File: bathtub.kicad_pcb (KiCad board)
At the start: 2 copper layers, 91.4 x 71.1 mm, 29 parts, among them J1 Screw_Terminal_01x03 - Hot wa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, J2 Screw_Terminal_01x03 - Cold w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, J3 Screw_Terminal_01x02, J4 Screw_Terminal_01x03 - Inputs, J5 Barrel_Jack, Q1 2N2219, Q2 2N2219, SW1 SW_Push, SW2 SW_Push

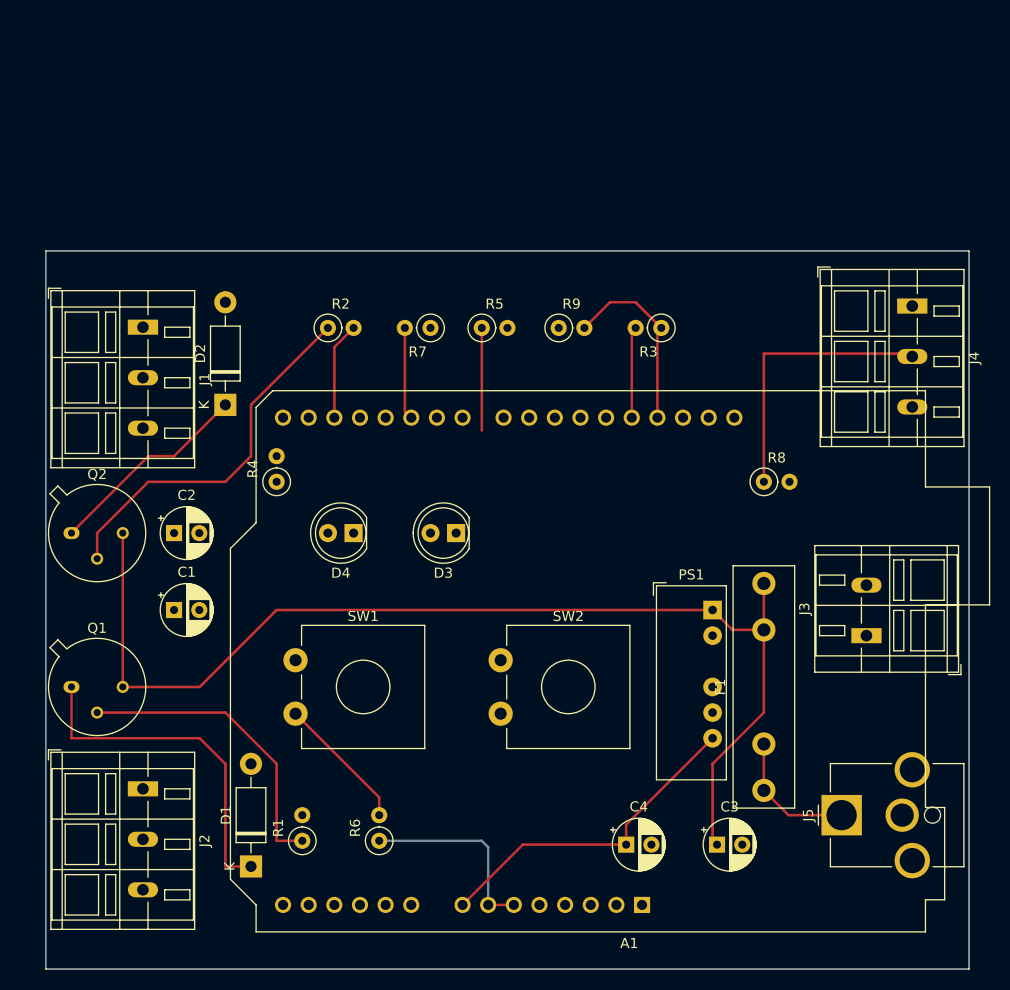
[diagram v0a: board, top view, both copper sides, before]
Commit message: feat: version 1.  Sent out for review
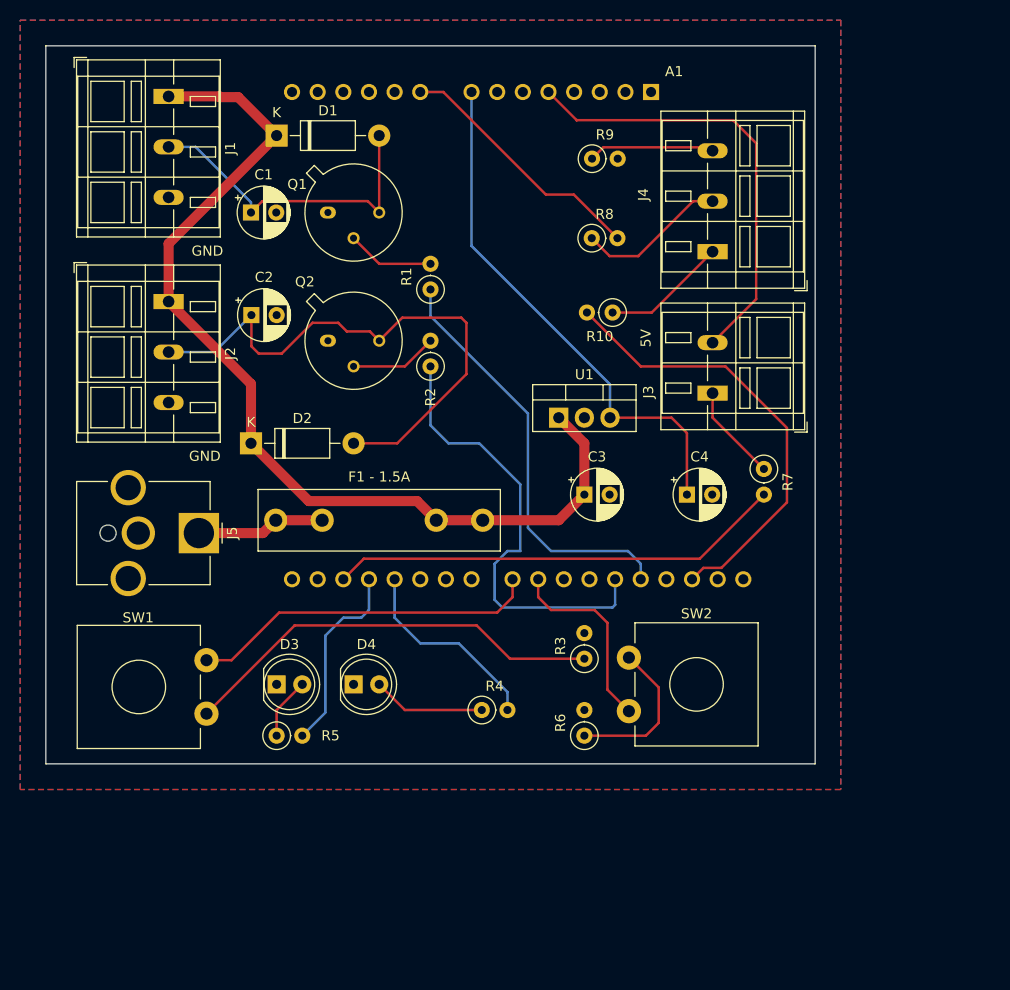
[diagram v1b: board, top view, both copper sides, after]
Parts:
- removed F1: Slow Blow Fuse - 1.5A, Fuse:Fuseholder_Littelfuse_100_series_5x20mm
- removed PS1: IH2405S, Converter_DCDC:Converter_DCDC_XP_POWER-IHxxxxS_THT
- added F1 - 1.5A: Slow Blow Fuse - 1.5A, Fuse:Fuseholder_Littelfuse_100_series_5x20mm, F.Cu at (119.3, 95.2)
- added R10: .01, Resistor_THT:R_Axial_DIN0207_L6.3mm_D2.5mm_P2.54mm_Vertical, F.Cu at (152.7, 74.7)
- added U1: L7805CV, Package_TO_SOT_THT:TO-220-3_Vertical, F.Cu at (147.3, 85.1)
- A1: moved to B.Cu
- C1, C2: value 0.1uF -> 0.01uF
- J1: value Screw_Terminal_01x03 - Hot water -> Screw_Terminal_01x03
- J2: value Screw_Terminal_01x03 - Cold water -> Screw_Terminal_01x03
- J3: value Screw_Terminal_01x02 -> Terminal_01x02
- J4: value Screw_Terminal_01x03 - Inputs -> Terminal 01x03 - Inputs
- R1, R2: value 250 ohms -> 250
- R3, R6: value 200ohm -> 200
- R4, R5: value 100ohm -> 220
- moved A1 80.5 mm to (156.5, 52.8)
- moved D1 72.4 mm to (119.4, 57.1), turned to 0 degrees
- moved J5 69.5 mm to (111.7, 96.5), turned to -90 degrees
- moved R1 56.1 mm to (134.6, 72.4)
- moved Q1 53.4 mm to (124.5, 64.8)
- moved J2 48.3 mm to (108.7, 73.6)
- moved R5 45.2 mm to (119.4, 116.6)
- moved C1 40.1 mm to (116.8, 64.8)
- moved C3 37.1 mm to (149.9, 92.7)
- moved R7 35.9 mm to (167.6, 90.2), turned to -90 degrees
- moved C4 35.2 mm to (160.0, 92.7)
- moved R3 33.6 mm to (149.9, 109.0), turned to 90 degrees
- moved Q2 31.7 mm to (124.5, 77.5)
- moved R4 30.4 mm to (139.7, 114.0), turned to 0 degrees
- moved R8 29.5 mm to (150.6, 67.3)
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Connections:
- net +5V renamed +12V
- A1 pad 20: Net-(A1-Pad20) -> unconnected-(A1-Pad20)
- A1 pad 21: Net-(A1-Pad21) -> unconnected-(A1-Pad21)
- A1 pad 24: unconnected-(A1-Pad24) -> Net-(A1-Pad24)
- A1 pad 27: unconnected-(A1-Pad27) -> Net-(A1-Pad27)
- A1 pad 29: -5V -> GND
- A1 pad 30: unconnected-(A1-Pad30) -> Net-(A1-Pad30)
- A1 pad 6: -5V -> GND
- A1 pad 7: -5V -> GND
- C1 pad 2: -24V -> GND
- C2 pad 1: Net-(C2-Pad1) -> Net-(D2-Pad2)
- C2 pad 2: -24V -> GND
- C3 pad 2: -24V -> GND
- C4 pad 2: -5V -> GND
- D1 pad 1: Net-(D1-Pad1) -> +24V
- D2 pad 1: Net-(D2-Pad1) -> +24V
- D2 pad 2: Net-(C2-Pad1) -> Net-(D2-Pad2)
- D3 pad 1: -5V -> GND
- D4 pad 1: -5V -> GND
- J1 pad 1: unconnected-(J1-Pad1) -> +24V
- J1 pad 2: unconnected-(J1-Pad2) -> Net-(C1-Pad1)
- J1 pad 3: -24V -> GND
- J2 pad 1: unconnected-(J2-Pad1) -> +24V
- J2 pad 2: unconnected-(J2-Pad2) -> Net-(D2-Pad2)
- J2 pad 3: -24V -> GND
- J3 pad 1: unconnected-(J3-Pad1) -> Net-(J3-Pad1)
- J3 pad 2: unconnected-(J3-Pad2) -> Net-(A1-Pad5)
- J4 pad 1: unconnected-(J4-Pad1) -> Net-(J4-Pad1)
- J4 pad 3: unconnected-(J4-Pad3) -> Net-(J4-Pad3)
- J5 pad 2: -24V -> GND
- Q1 pad 1: Net-(D1-Pad1) -> GND
- Q1 pad 3: +24V -> Net-(C1-Pad1)
- Q2 pad 1: Net-(D2-Pad1) -> GND
- Q2 pad 3: +24V -> Net-(D2-Pad2)
- R1 pad 1: Net-(Q1-Pad2) -> Net-(A1-Pad28)
- R1 pad 2: Net-(A1-Pad21) -> Net-(Q1-Pad2)
- R2 pad 1: Net-(Q2-Pad2) -> Net-(A1-Pad27)
- R2 pad 2: Net-(A1-Pad17) -> Net-(Q2-Pad2)
- R3 pad 1: -5V -> Net-(R3-Pad1)
- R3 pad 2: Net-(A1-Pad28) -> GND
- R6 pad 1: -5V -> Net-(R6-Pad1)
- R6 pad 2: Net-(A1-Pad23) -> GND
- R7 pad 1: unconnected-(R7-Pad1) -> Net-(J3-Pad1)
- R7 pad 2: Net-(A1-Pad20) -> Net-(A1-Pad17)
- R9 pad 1: unconnected-(R9-Pad1) -> Net-(J4-Pad3)
- R9 pad 2: -5V -> GND
- SW1 pad 1: Net-(A1-Pad5) -> Net-(R3-Pad1)
- SW2 pad 1: Net-(A1-Pad5) -> Net-(R6-Pad1)
- SW2 pad 2: Net-(A1-Pad28) -> Net-(A1-Pad24)
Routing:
- net Net-(D2-Pad2): track 0.00 -> 56.7 mm
- net Net-(A1-Pad27): track 0.00 -> 45.3 mm
- net Net-(A1-Pad30): track 0.00 -> 44.5 mm
- net Net-(A1-Pad5): track 0.00 -> 44.2 mm
- net Net-(R3-Pad1): track 0.00 -> 42.4 mm
- net -5V: track 38.1 -> 0.00 mm
- net Net-(A1-Pad17): track 9.68 -> 45.1 mm
- net Net-(D1-Pad1): track 34.1 -> 0.00 mm
- net Net-(A1-Pad28): track 9.05 -> 41.8 mm
- net Net-(C1-Pad1): track 0.00 -> 32.7 mm
- net Net-(Q2-Pad2): track 36.8 -> 8.67 mm
- net Net-(A1-Pad9): track 0.00 -> 25.5 mm
- net Net-(Q1-Pad2): track 30.0 -> 8.67 mm
- net Net-(A1-Pad23): track 13.5 -> 34.7 mm
- net Net-(D2-Pad1): track 20.5 -> 0.00 mm
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- added copper zone on B.Cu, net GND
- added copper zone on F.Cu, net GND
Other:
- board size 91.4 x 71.1 mm -> 76.2 x 71.1 mm
- board text added: "5V"
- board text added: "GND"
